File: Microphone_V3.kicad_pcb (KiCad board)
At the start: 2 copper layers, 91.4 x 61 mm, 5 parts

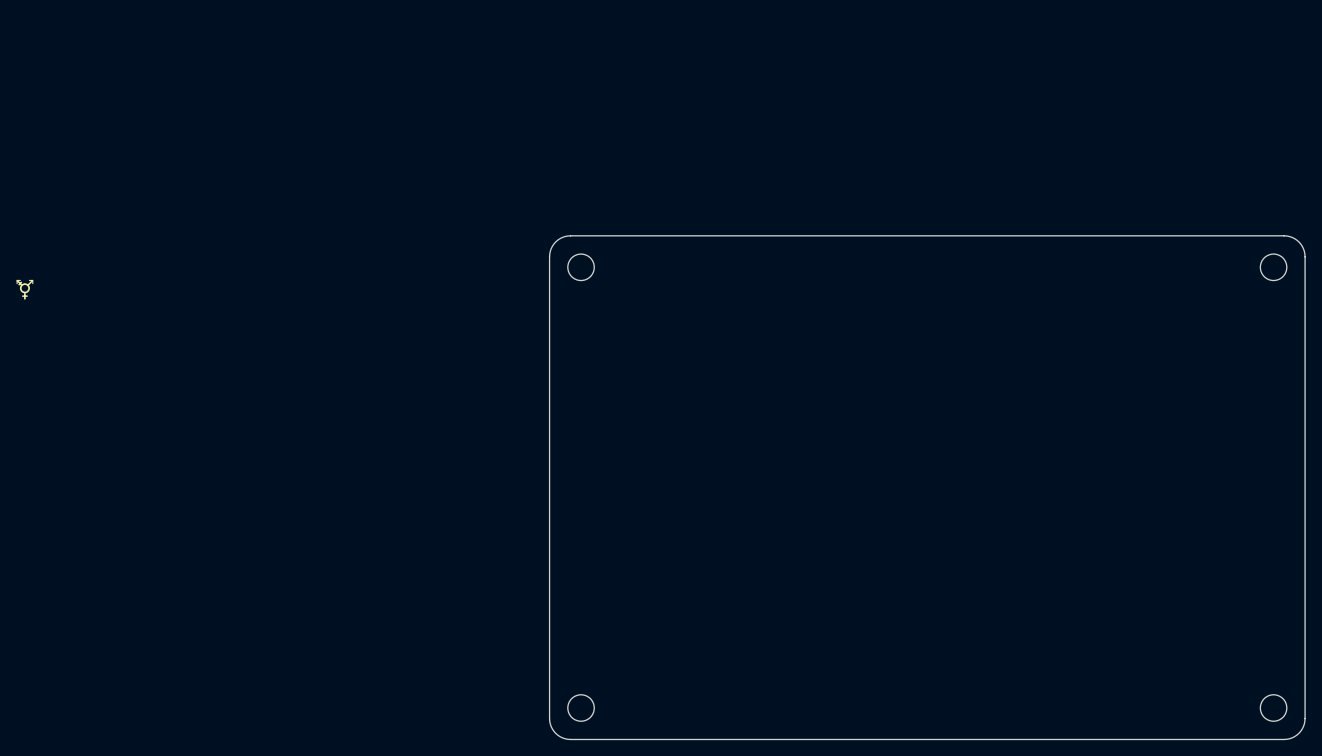
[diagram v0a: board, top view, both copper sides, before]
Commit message: layout
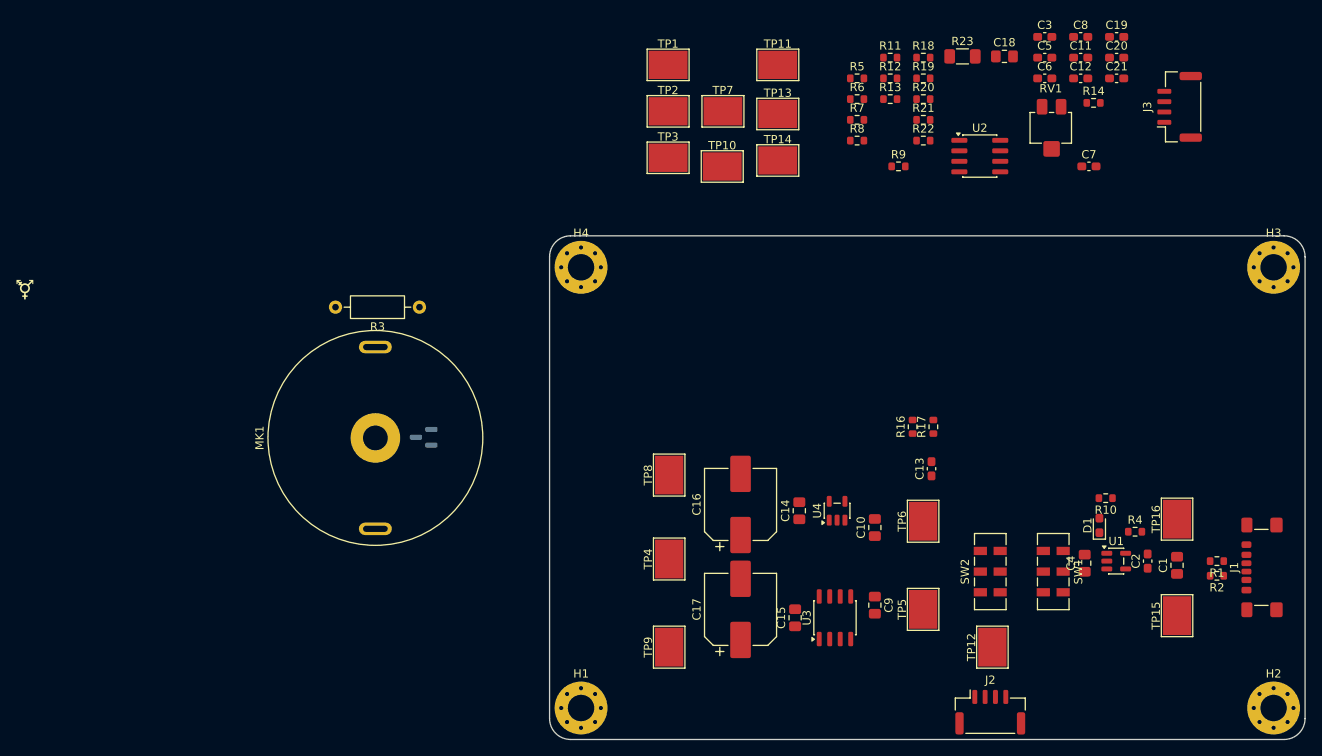
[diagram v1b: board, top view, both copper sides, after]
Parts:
- added C1: 10uF, Capacitor_SMD:C_0805_2012Metric_Pad1.18x1.45mm_HandSolder, F.Cu at (195.3, 100.8)
- added C10: 10uF, Capacitor_SMD:C_0805_2012Metric_Pad1.18x1.45mm_HandSolder, F.Cu at (158.8, 96.3)
- added C11: 24nF, Capacitor_SMD:C_0603_1608Metric_Pad1.08x0.95mm_HandSolder, F.Cu at (183.7, 39.4)
- added C12: 24nF, Capacitor_SMD:C_0603_1608Metric_Pad1.08x0.95mm_HandSolder, F.Cu at (183.7, 41.9)
- added C13: 0.01uF, Capacitor_SMD:C_0603_1608Metric_Pad1.08x0.95mm_HandSolder, F.Cu at (165.6, 89.2)
- added C14: 10uF, Capacitor_SMD:C_0805_2012Metric_Pad1.18x1.45mm_HandSolder, F.Cu at (149.6, 94.2)
- added C15: 10uF, Capacitor_SMD:C_0805_2012Metric_Pad1.18x1.45mm_HandSolder, F.Cu at (149.1, 107.2)
- added C16: 100uF, Capacitor_SMD:CP_Elec_8x10.5, F.Cu at (142.5, 93.5)
- added C17: 100uF, Capacitor_SMD:CP_Elec_8x10.5, F.Cu at (142.5, 106.2)
- added C18: 10uF, Capacitor_SMD:C_0805_2012Metric_Pad1.18x1.45mm_HandSolder, F.Cu at (174.4, 39.2)
- added C19: 22nF, Capacitor_SMD:C_0603_1608Metric_Pad1.08x0.95mm_HandSolder, F.Cu at (188.0, 36.9)
- added C2: 0.1uF, Capacitor_SMD:C_0603_1608Metric_Pad1.08x0.95mm_HandSolder, F.Cu at (191.8, 100.3)
- added C20: 22nF, Capacitor_SMD:C_0603_1608Metric_Pad1.08x0.95mm_HandSolder, F.Cu at (188.0, 39.4)
- added C21: 22nF, Capacitor_SMD:C_0603_1608Metric_Pad1.08x0.95mm_HandSolder, F.Cu at (188.0, 41.9)
- added C3: 22nF, Capacitor_SMD:C_0603_1608Metric_Pad1.08x0.95mm_HandSolder, F.Cu at (179.3, 36.9)
- added C4: 10uF, Capacitor_SMD:C_0805_2012Metric_Pad1.18x1.45mm_HandSolder, F.Cu at (184.2, 100.6)
- added C5: 22nF, Capacitor_SMD:C_0603_1608Metric_Pad1.08x0.95mm_HandSolder, F.Cu at (179.3, 39.4)
- added C6: 0.1uF, Capacitor_SMD:C_0603_1608Metric_Pad1.08x0.95mm_HandSolder, F.Cu at (179.3, 41.9)
- added C7: 0.1uF, Capacitor_SMD:C_0603_1608Metric_Pad1.08x0.95mm_HandSolder, F.Cu at (184.7, 52.6)
- added C8: 1nF, Capacitor_SMD:C_0603_1608Metric_Pad1.08x0.95mm_HandSolder, F.Cu at (183.7, 36.9)
- added C9: 10uF, Capacitor_SMD:C_0805_2012Metric_Pad1.18x1.45mm_HandSolder, F.Cu at (158.8, 105.7)
- added D1: LED, LED_SMD:LED_0603_1608Metric_Pad1.05x0.95mm_HandSolder, F.Cu at (185.9, 96.0)
- added J1: USB4135-GF-A, Connector_USB:USB_C_Receptacle_GCT_USB4135-GF-A_6P_TopMnt_Horizontal, F.Cu at (206.8, 101.1)
- added J2: SM04B-GHS-TB, Connector_JST:JST_GH_SM04B-GHS-TB_1x04-1MP_P1.25mm_Horizontal, F.Cu at (172.7, 118.6)
- added J3: SM04B-GHS-TB, Connector_JST:JST_GH_SM04B-GHS-TB_1x04-1MP_P1.25mm_Horizontal, F.Cu at (195.6, 45.3)
- added MK1: JLI-2555BXZ3-GP, jannett_footprints:JLI-2555BXZ3-GP, F.Cu at (98.3, 85.4)
- added Q1: SST4416, Package_TO_SOT_SMD:SOT-23, B.Cu at (104.1, 85.3)
- added R1: 5.11K, Resistor_SMD:R_0603_1608Metric, F.Cu at (200.2, 100.3)
- added R10: 1K, Resistor_SMD:R_0603_1608Metric, F.Cu at (186.7, 92.7)
- added R11: 0, Resistor_SMD:R_0603_1608Metric, F.Cu at (160.6, 39.4)
- added R12: 0, Resistor_SMD:R_0603_1608Metric, F.Cu at (160.6, 41.9)
- added R13: 95.3K, Resistor_SMD:R_0603_1608Metric, F.Cu at (160.6, 44.4)
- added R14: 1K, Resistor_SMD:R_0603_1608Metric, F.Cu at (185.2, 44.9)
- added R16: 0, Resistor_SMD:R_0603_1608Metric, F.Cu at (163.3, 84.1)
- added R17: 0, Resistor_SMD:R_0603_1608Metric, F.Cu at (165.8, 84.1)
- added R18: 69.8K, Resistor_SMD:R_0603_1608Metric, F.Cu at (164.6, 39.4)
- added R19: 133K, Resistor_SMD:R_0603_1608Metric, F.Cu at (164.6, 41.9)
- added R2: 5.11K, Resistor_SMD:R_0603_1608Metric, F.Cu at (200.2, 102.1)
- added R20: 0, Resistor_SMD:R_0603_1608Metric, F.Cu at (164.6, 44.4)
- added R21: 0, Resistor_SMD:R_0603_1608Metric, F.Cu at (164.6, 46.9)
- added R22: 1MEG, Resistor_SMD:R_0603_1608Metric, F.Cu at (164.6, 49.4)
- added R23: 5.11MEG, Resistor_SMD:R_1206_3216Metric_Pad1.30x1.75mm_HandSolder, F.Cu at (169.4, 39.2)
- added R3: 1G, Resistor_THT:R_Axial_DIN0207_L6.3mm_D2.5mm_P10.16mm_Horizontal, F.Cu at (103.6, 69.6)
- added R4: 2K, Resistor_SMD:R_0603_1608Metric, F.Cu at (190.2, 96.8)
- added R5: 0, Resistor_SMD:R_0603_1608Metric, F.Cu at (156.6, 41.9)
- added R6: 4.7K, Resistor_SMD:R_0603_1608Metric, F.Cu at (156.6, 44.4)
- added R7: 2.21K, Resistor_SMD:R_0603_1608Metric, F.Cu at (156.6, 46.9)
- added R8: 0, Resistor_SMD:R_0603_1608Metric, F.Cu at (156.6, 49.4)
- added R9: 1K, Resistor_SMD:R_0603_1608Metric, F.Cu at (161.6, 52.6)
- added RV1: 3214X-1-103E, Potentiometer_SMD:Potentiometer_Bourns_3214X_Vertical, F.Cu at (180.1, 47.9)
- added SW1: JS202011JCQN, jannett_footprints:SW_DPDT_CK_JS202011JCQN, F.Cu at (180.3, 101.6)
- added SW2: JS202011JCQN, jannett_footprints:SW_DPDT_CK_JS202011JCQN, F.Cu at (172.7, 101.6)
- added TP1: 5016, jannett_footprints:TestPoint_Keystone_5016_Compact, F.Cu at (133.7, 40.3)
- added TP10: 5016, jannett_footprints:TestPoint_Keystone_5016_Compact, F.Cu at (140.3, 52.6)
- added TP11: 5016, jannett_footprints:TestPoint_Keystone_5016_Compact, F.Cu at (147.0, 40.3)
- added TP12: 5016, jannett_footprints:TestPoint_Keystone_5016_Compact, F.Cu at (173.0, 110.7)
- added TP13: 5016, jannett_footprints:TestPoint_Keystone_5016_Compact, F.Cu at (147.0, 46.2)
- added TP14: 5016, jannett_footprints:TestPoint_Keystone_5016_Compact, F.Cu at (147.0, 51.8)
- added TP15: 5016, jannett_footprints:TestPoint_Keystone_5016_Compact, F.Cu at (195.3, 106.9)
- added TP16: 5016, jannett_footprints:TestPoint_Keystone_5016_Compact, F.Cu at (195.3, 95.2)
- added TP2: 5016, jannett_footprints:TestPoint_Keystone_5016_Compact, F.Cu at (133.7, 45.9)
- added TP3: 5016, jannett_footprints:TestPoint_Keystone_5016_Compact, F.Cu at (133.7, 51.5)
- added TP4: 5016, jannett_footprints:TestPoint_Keystone_5016_Compact, F.Cu at (133.9, 100.1)
- added TP5: 5016, jannett_footprints:TestPoint_Keystone_5016_Compact, F.Cu at (164.6, 106.2)
- added TP6: 5016, jannett_footprints:TestPoint_Keystone_5016_Compact, F.Cu at (164.6, 95.5)
- added TP7: 5016, jannett_footprints:TestPoint_Keystone_5016_Compact, F.Cu at (140.4, 45.9)
- added TP8: 5016, jannett_footprints:TestPoint_Keystone_5016_Compact, F.Cu at (133.9, 89.9)
- added TP9: 5016, jannett_footprints:TestPoint_Keystone_5016_Compact, F.Cu at (133.9, 110.7)
- added U1: MCP73831-2-OT, Package_TO_SOT_SMD:SOT-23-5, F.Cu at (188.0, 100.3)
- added U2: AD8616ARZ, Package_SO:SOIC-8_3.9x4.9mm_P1.27mm, F.Cu at (171.4, 51.3)
- added U3: LT1763CS8-2.5#PBF, Package_SO:SO-8_3.9x4.9mm_P1.27mm, F.Cu at (153.9, 107.2)
- added U4: ADP7182AUJZ-2.5, Package_TO_SOT_SMD:TSOT-23-5, F.Cu at (154.2, 94.2)
- H1, H2, H3, H4: footprint MountingHole:MountingHole_3.2mm_M3_ISO14580 -> MountingHole:MountingHole_3.2mm_M3_Pad_Via
- SYMBOL1: footprint Jarrett_Footprint_Library:Trans_Symbol -> jannett_footprints:Trans_Symbol
